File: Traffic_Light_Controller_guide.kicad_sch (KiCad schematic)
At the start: 64 parts, among them J1 Conn_02x08_Odd_Even, J2 Conn_02x08_Odd_Even, J3 Conn_02x05_Odd_Even, J4 +5V, SW1 SW_Push, SW2 OVR, SW3 EN, U1 SM420561N, U2 SM420561N, U3 LM1117DT-3.3

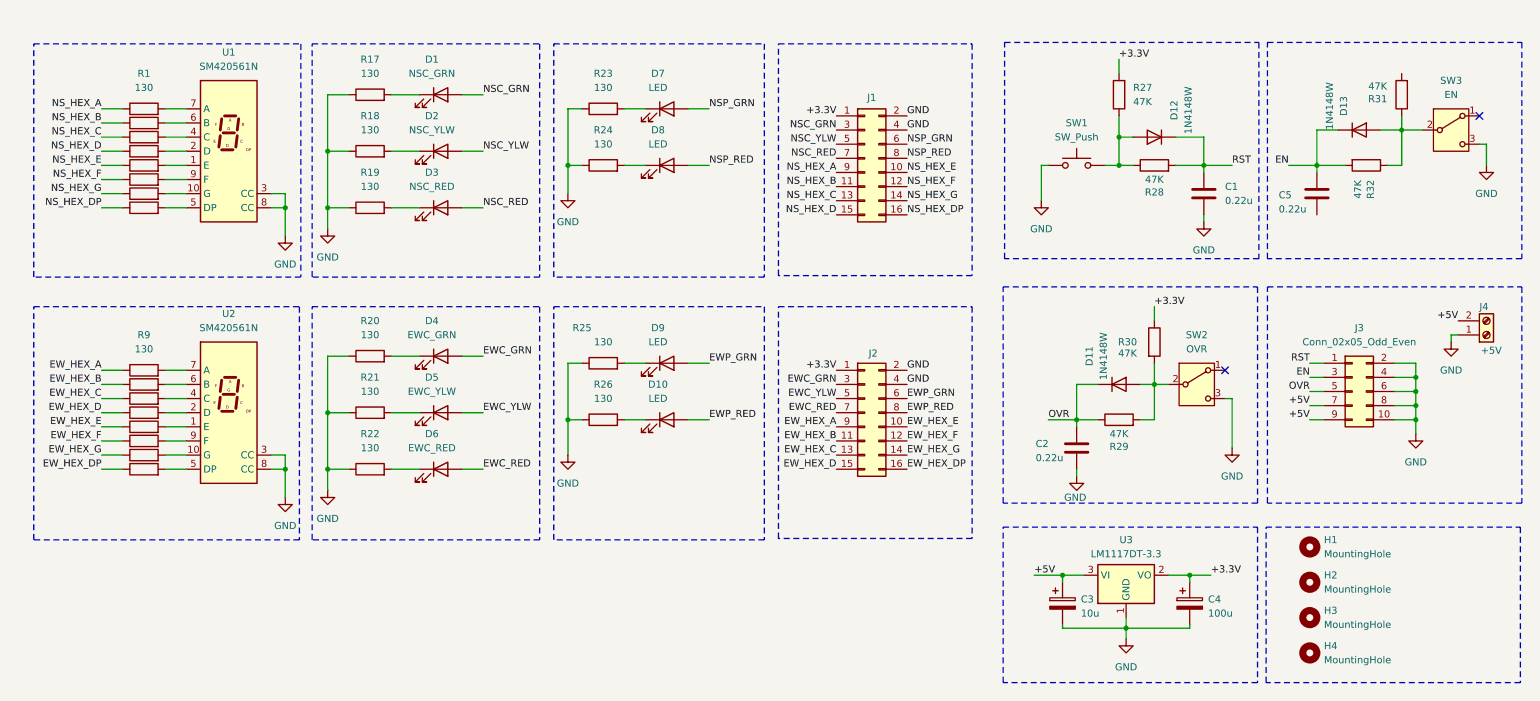
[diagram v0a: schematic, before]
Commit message: FINISH EXAM
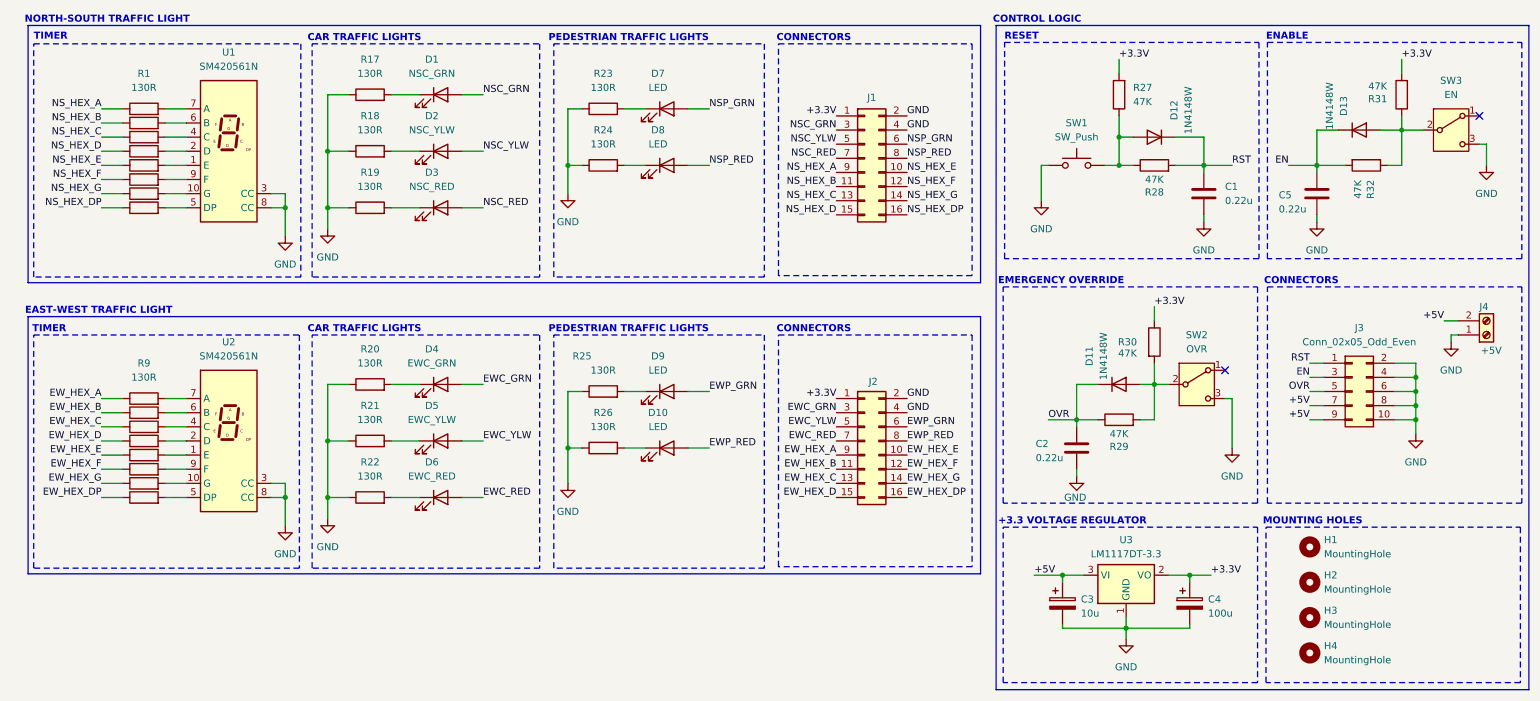
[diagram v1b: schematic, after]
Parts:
- C3: footprint Capacitor_SMD:CP_Elec_6.3x3 -> Capacitor_SMD:CP_Elec_4x5.3
- C4: footprint Capacitor_SMD:CP_Elec_6.3x3 -> Capacitor_SMD:CP_Elec_6.3x5.8
- C5: footprint Capacitor_SMD:C_1206_3216Metric_Pad1.33x1.80mm_HandSolder -> LED_SMD:LED_1206_3216Metric_Pad1.42x1.75mm_HandSolder
- D1, D2, D3, D4, D5, D6: footprint Diode_SMD:D_1206_3216Metric_Pad1.42x1.75mm_HandSolder -> LED_THT:LED_D5.0mm
- D10, D7, D8, D9: footprint LED_SMD:LED_1206_3216Metric_Pad1.42x1.75mm_HandSolder -> LED_THT:LED_D5.0mm
- R1, R17, R18, R19, R20, R21, R22, R23, R24, R25, R26, R9: value 130 -> 130R
- U3: footprint Package_TO_SOT_SMD:TO-252-3_TabPin2 -> Package_TO_SOT_SMD:SOT-223-3_TabPin2
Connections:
- net +3.3V: now also R31.2
- net GND: now also C5.2
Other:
- note added: "+3.3 VOLTAGE REGULATOR"
- note added: "CAR TRAFFIC LIGHTS"
- note added: "CONNECTORS"
- note added: "CONTROL LOGIC"
- note added: "EAST-WEST TRAFFIC LIGHT"
- note added: "EMERGENCY OVERRIDE"
- note added: "ENABLE"
- note added: "MOUNTING HOLES"
- note added: "NORTH-SOUTH TRAFFIC LIGHT"
- note added: "PEDESTRIAN TRAFFIC LIGHTS"
- note added: "RESET"
- note added: "TIMER"
- moved on the sheet: D10, D4, D5, D6, D9, J2, R20, R21, R22, R25, R26, R9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
